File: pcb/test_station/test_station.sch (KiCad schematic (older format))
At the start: 10 parts

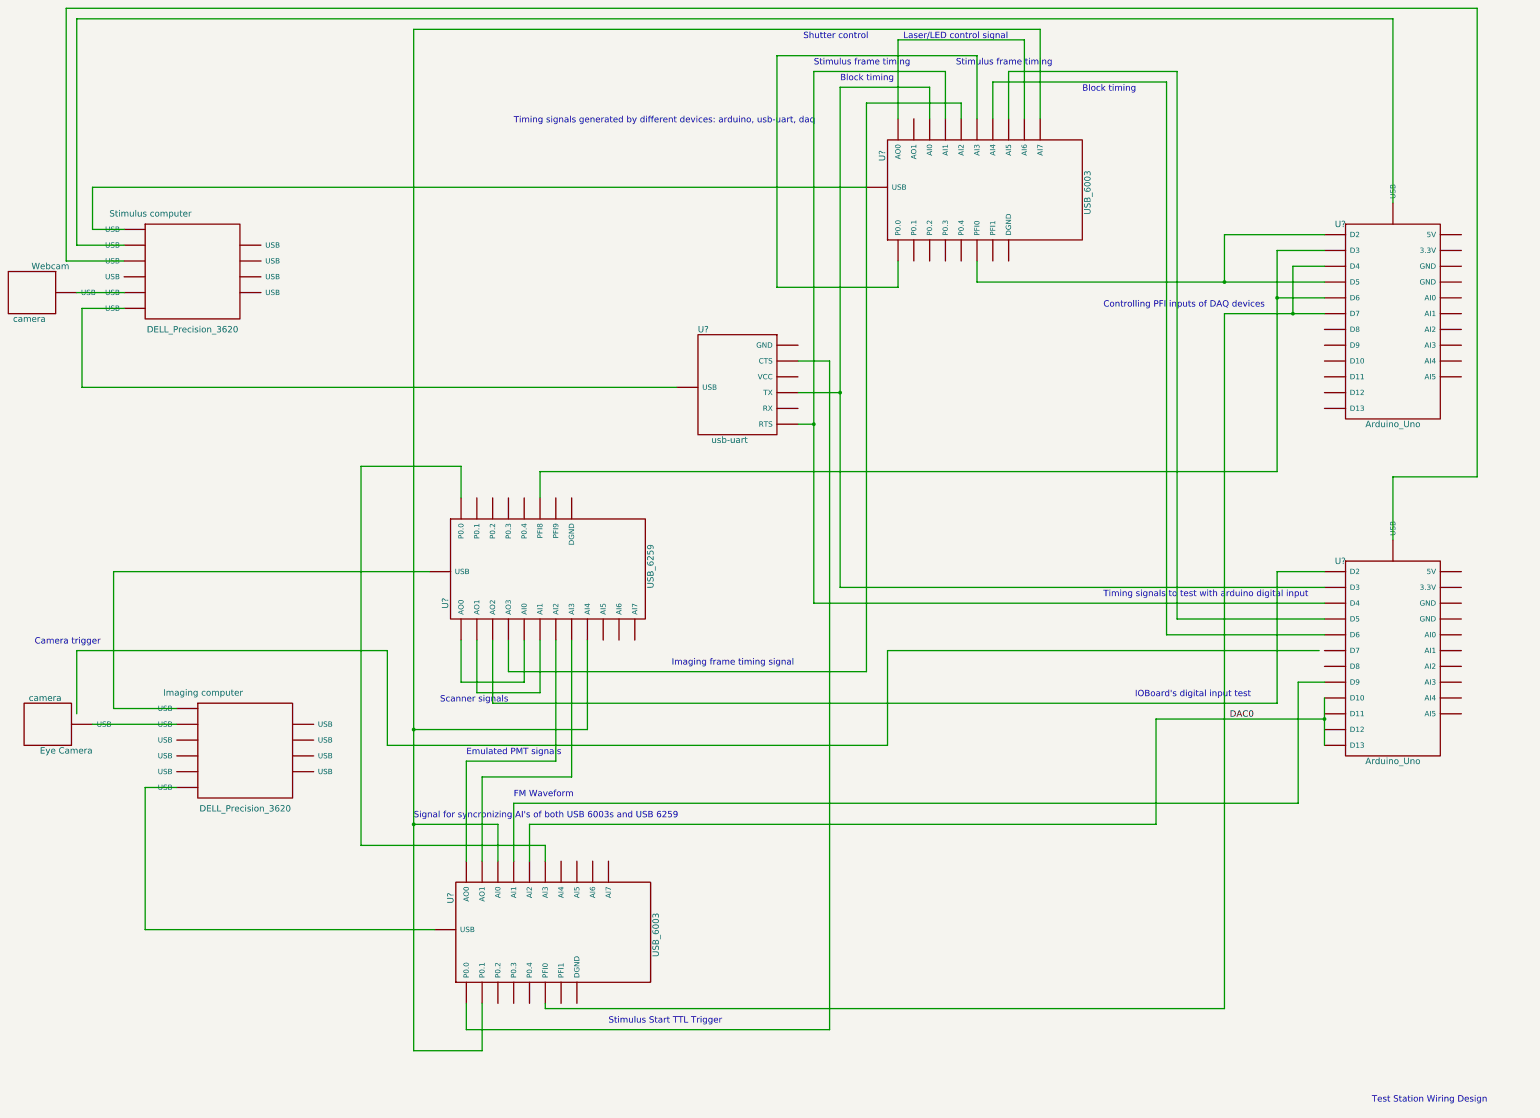
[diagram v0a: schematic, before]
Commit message: Test station design rewired
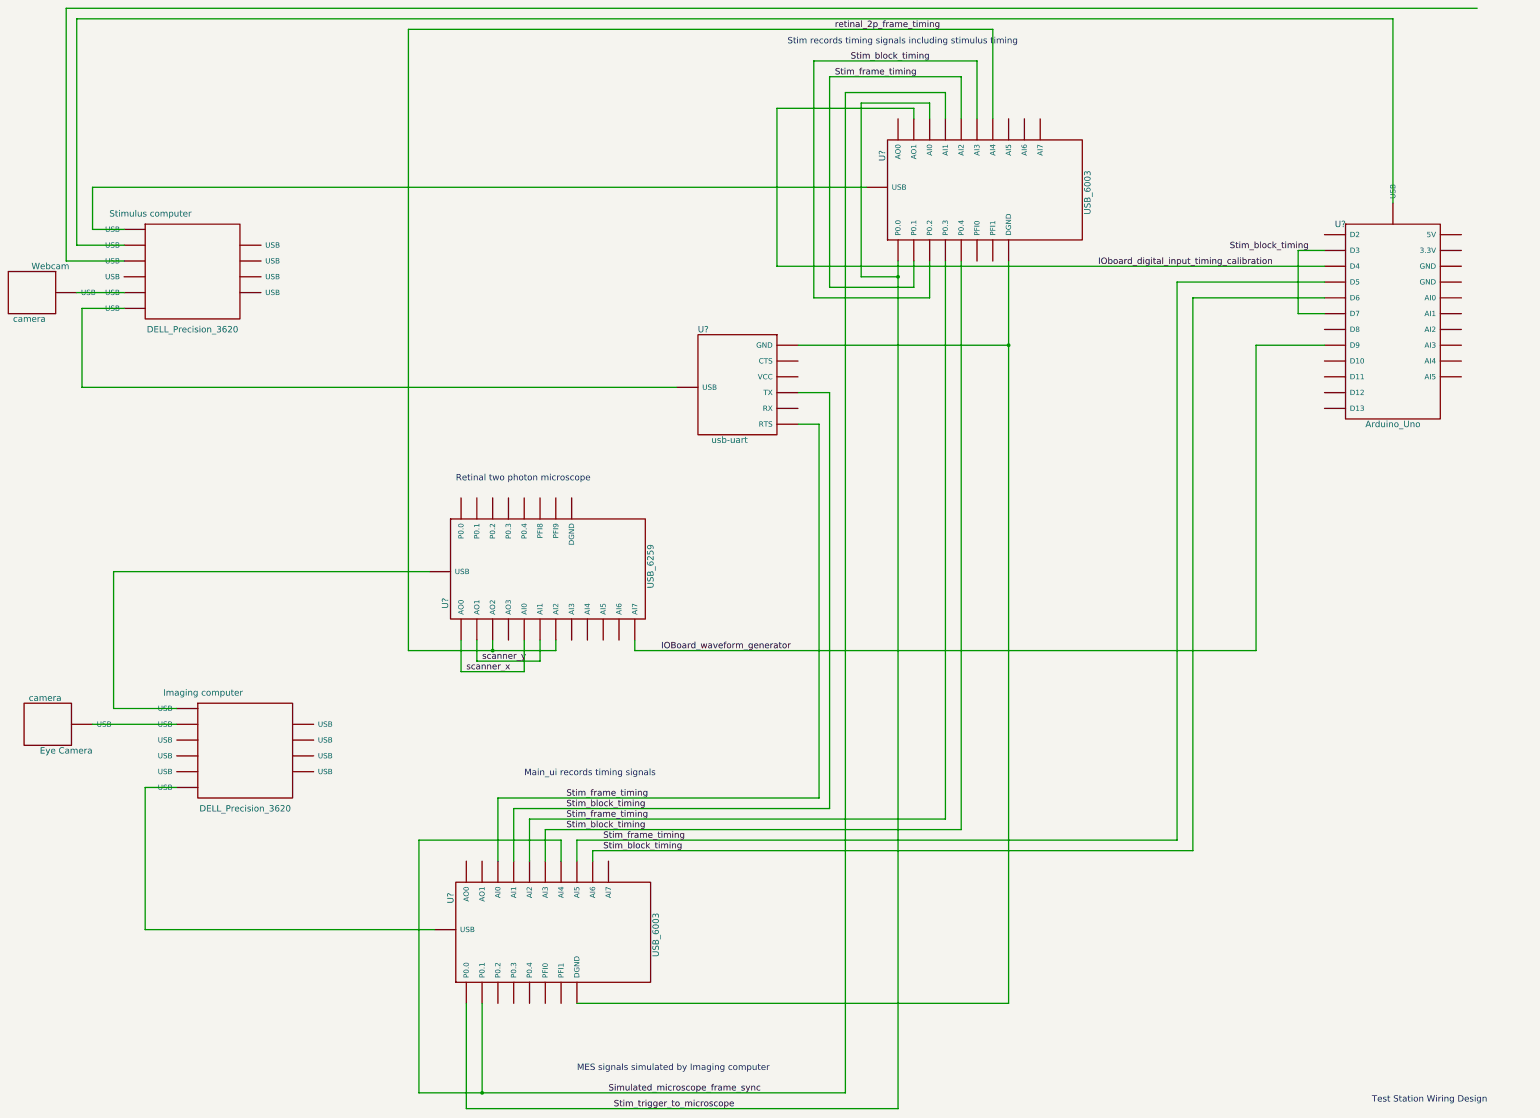
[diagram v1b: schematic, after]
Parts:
- removed U?: Arduino_Uno, symbol Arduino_Uno
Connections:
- net labels added: IOBoard_waveform_generator, IOboard_digital_input_timing_calibration, Simulated_microscope_frame_sync, Stim_block_timing, Stim_frame_timing, Stim_trigger_to_microscope, retinal_2p_frame_timing, scanner_x, scanner_y
- net labels removed: DAC0
- wire segments 119 -> 94
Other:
- note added: "MES signals simulated by Imaging computer"
- note added: "Main_ui records timing signals"
- note added: "Retinal two photon microscope"
- note added: "Stim records timing signals including stimulus timing"
- note removed: "Block timing"
- note removed: "Camera trigger"
- note removed: "Controlling PFI inputs of DAQ devices"
- note removed: "Emulated PMT signals"
- note removed: "FM Waveform"
- note removed: "IOBoard's digital input test"
- note removed: "Imaging frame timing signal"
- note removed: "Laser/LED control signal"
- note removed: "Scanner signals"
- note removed: "Shutter control"
- note removed: "Signal for syncronizing AI's of both USB 6003s and USB 6259"
- note removed: "Stimulus Start TTL Trigger"
- note removed: "Stimulus frame timing"
- note removed: "Timing signals generated by different devices: arduino, usb-uart, daq"
- note removed: "Timing signals to test with arduino digital input"
